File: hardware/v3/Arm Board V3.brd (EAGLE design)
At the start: 114.3 x 76.2 mm, 83 parts, among them CN1 1X4-BIG, IC1 L6208D, IC10 74LVC1G125DCK, IC2 L6208D, IC3 L6208D, IC4 LMV358IDGKR, IC5 NCP1117ST33T3G -3V3, IC6 ATMEGA16U2-MU, Q2 BC847BSMD, T1 FDN340P, T2 FDN340P, T3 FDN340P, U2 ST3485EBDR, U3 ATSAM3X8EA-AU, Y1 12MHz KX-7 20pF, Y2 32.768Khz, Y4 12MHz KX-7 20pF

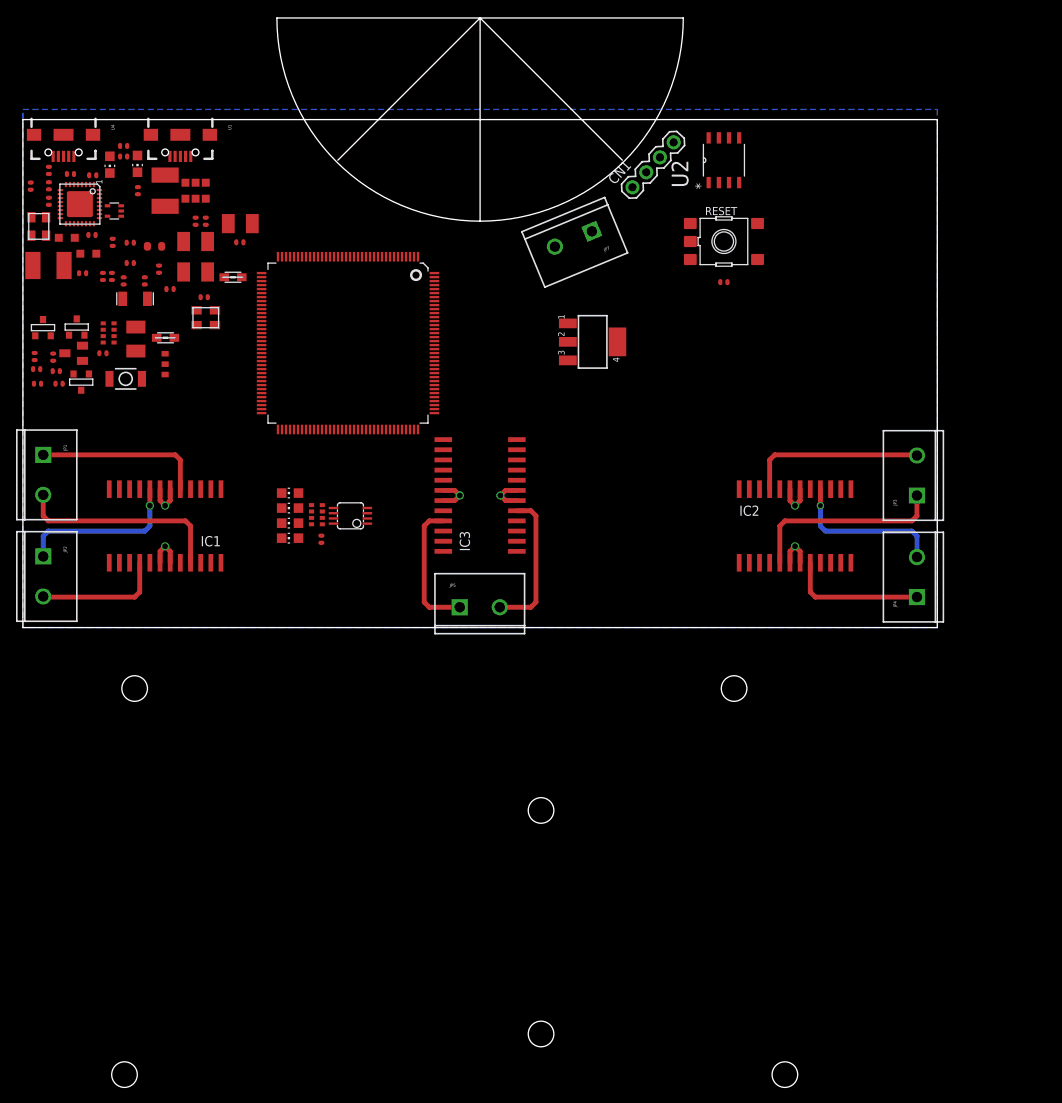
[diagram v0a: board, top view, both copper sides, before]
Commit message: XBEE
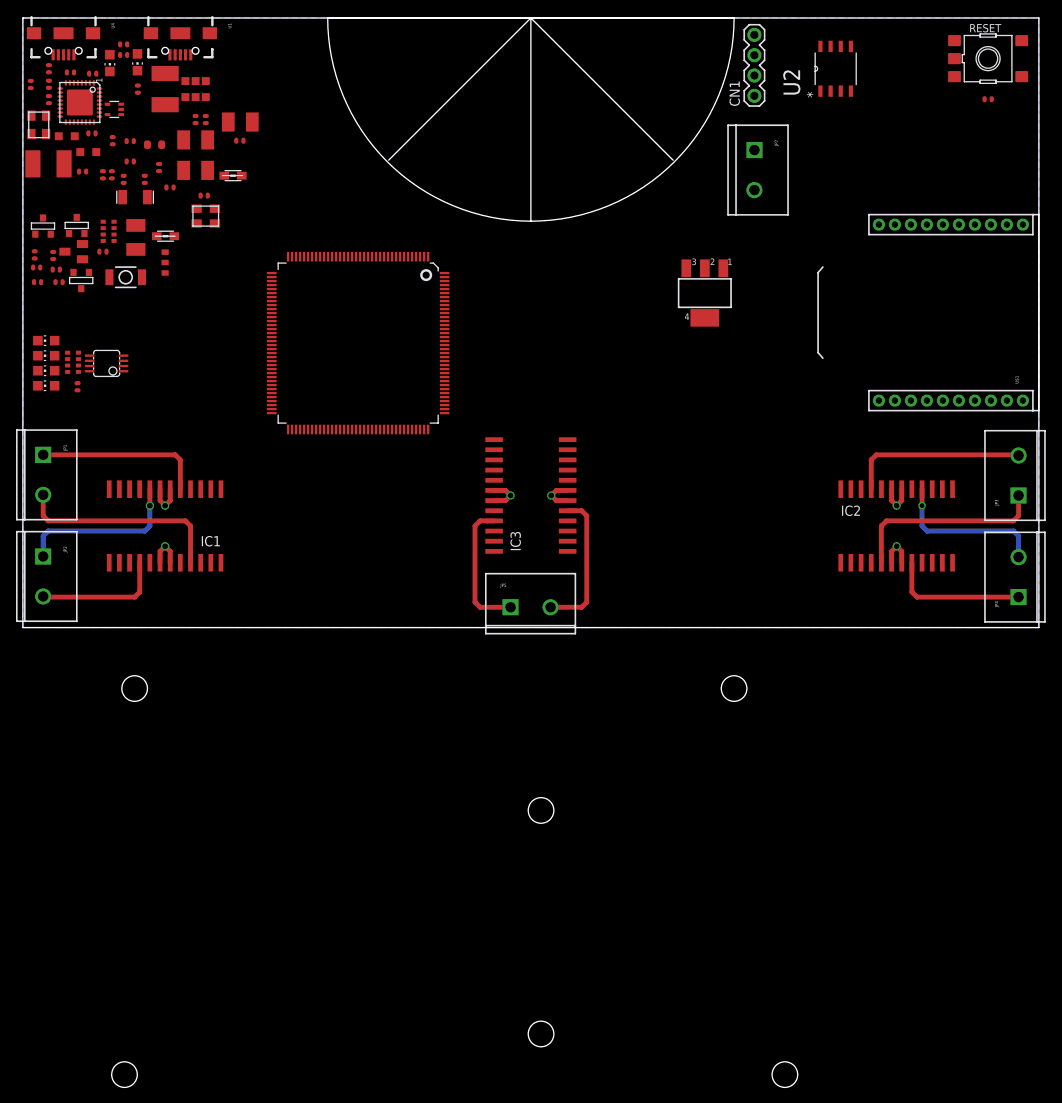
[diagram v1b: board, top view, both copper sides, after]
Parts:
- added U$1: XBEE-1B2, SparkFun-RF:XBEE-SILK
- moved C20 40.2 mm to (120.7, 66.0)
- moved RESET 40.2 mm to (120.7, 71.1)
- moved L 35.9 mm to (2.92, 32.1)
- moved C30 35.9 mm to (6.83, 30.1)
- moved IC4 35.9 mm to (10.5, 33.0)
- moved ON 35.9 mm to (2.92, 30.2)
- moved RX 35.9 mm to (2.92, 35.9)
- moved TX 35.9 mm to (2.92, 34.0)
- moved RN3 35.9 mm to (6.27, 33.2)
- moved JP7 22.7 mm to (91.4, 59.7), turned to 270 degrees
- moved CN1 19.0 mm to (91.4, 66.5), turned to 90 degrees
- moved U2 18.1 mm to (101.6, 69.8)
- moved IC5 15.3 mm to (85.2, 41.8), turned to 180 degrees
- moved C23 12.7 mm to (12.6, 56.0)
- moved C24 12.7 mm to (15.2, 56.0)
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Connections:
- new net VDD: U$1.1
- net GND: now also U$1.10
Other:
- board size 114.3 x 76.2 mm -> 127 x 76.2 mm
